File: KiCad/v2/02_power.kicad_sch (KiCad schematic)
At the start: 45 parts, among them IC201 TPS63000DRCR, IC202 TPS63000DRCR, J201 Barrel_Jack_Switch_Pin3Ring, J202 Conn_01x03_Pin, J203 Conn_02x03_Odd_Even, J204 Conn_01x03_Pin, J205 Conn_02x03_Odd_Even

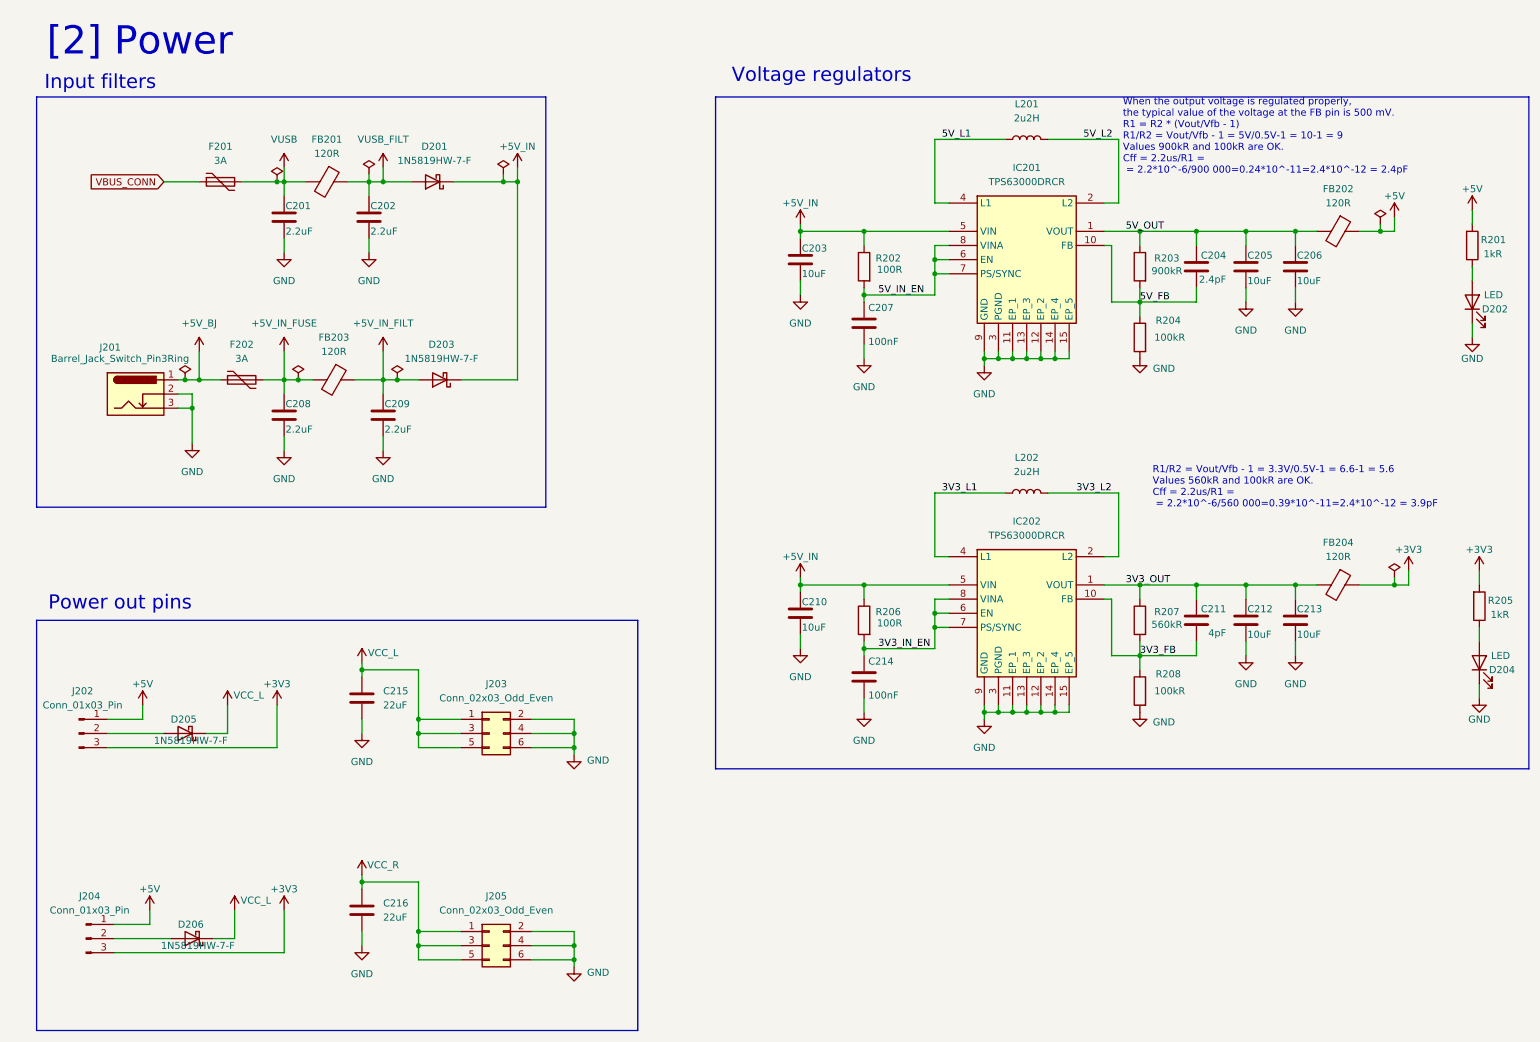
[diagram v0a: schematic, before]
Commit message: Initial components placement
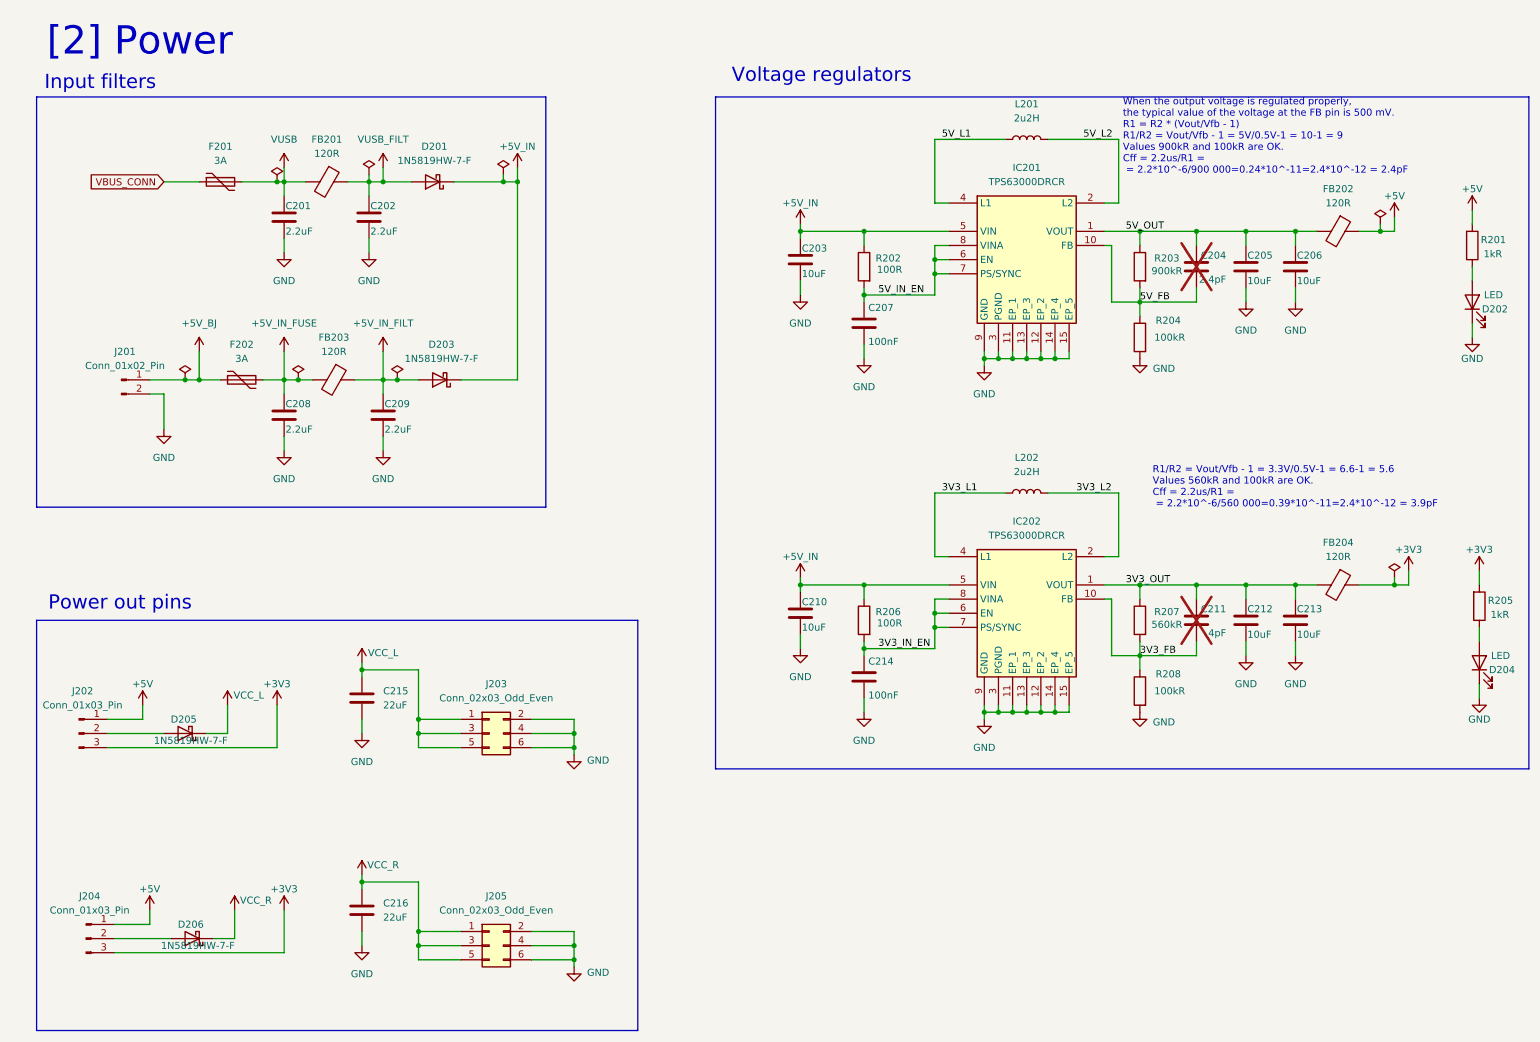
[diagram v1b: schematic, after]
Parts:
- removed J201: Barrel_Jack_Switch_Pin3Ring, Connector_BarrelJack:BarrelJack_GCT_DCJ200-10-A_Horizontal, symbol Connector:Barrel_Jack_Switch_Pin3Ring
- added J201: Conn_01x02_Pin, Connector_PinHeader_2.54mm:PinHeader_1x02_P2.54mm_Vertical, symbol Connector:Conn_01x02_Pin
- C204, C211: now not fitted
- C207, C214: footprint Capacitor_SMD:C_0603_1608Metric -> Capacitor_SMD:C_0402_1005Metric
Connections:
- net +5V_BJ: now also J201.1 (Pin_1)
- net GND: now also J201.2 (Pin_2)
- net VCC_L: no longer D206.1 (K)
- net VCC_R: now also D206.1 (K)
